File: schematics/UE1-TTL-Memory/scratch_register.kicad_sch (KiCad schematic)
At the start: 9 parts, among them U1 74LS139, U2 74LS259, U3 74LS151, U4 74LS125

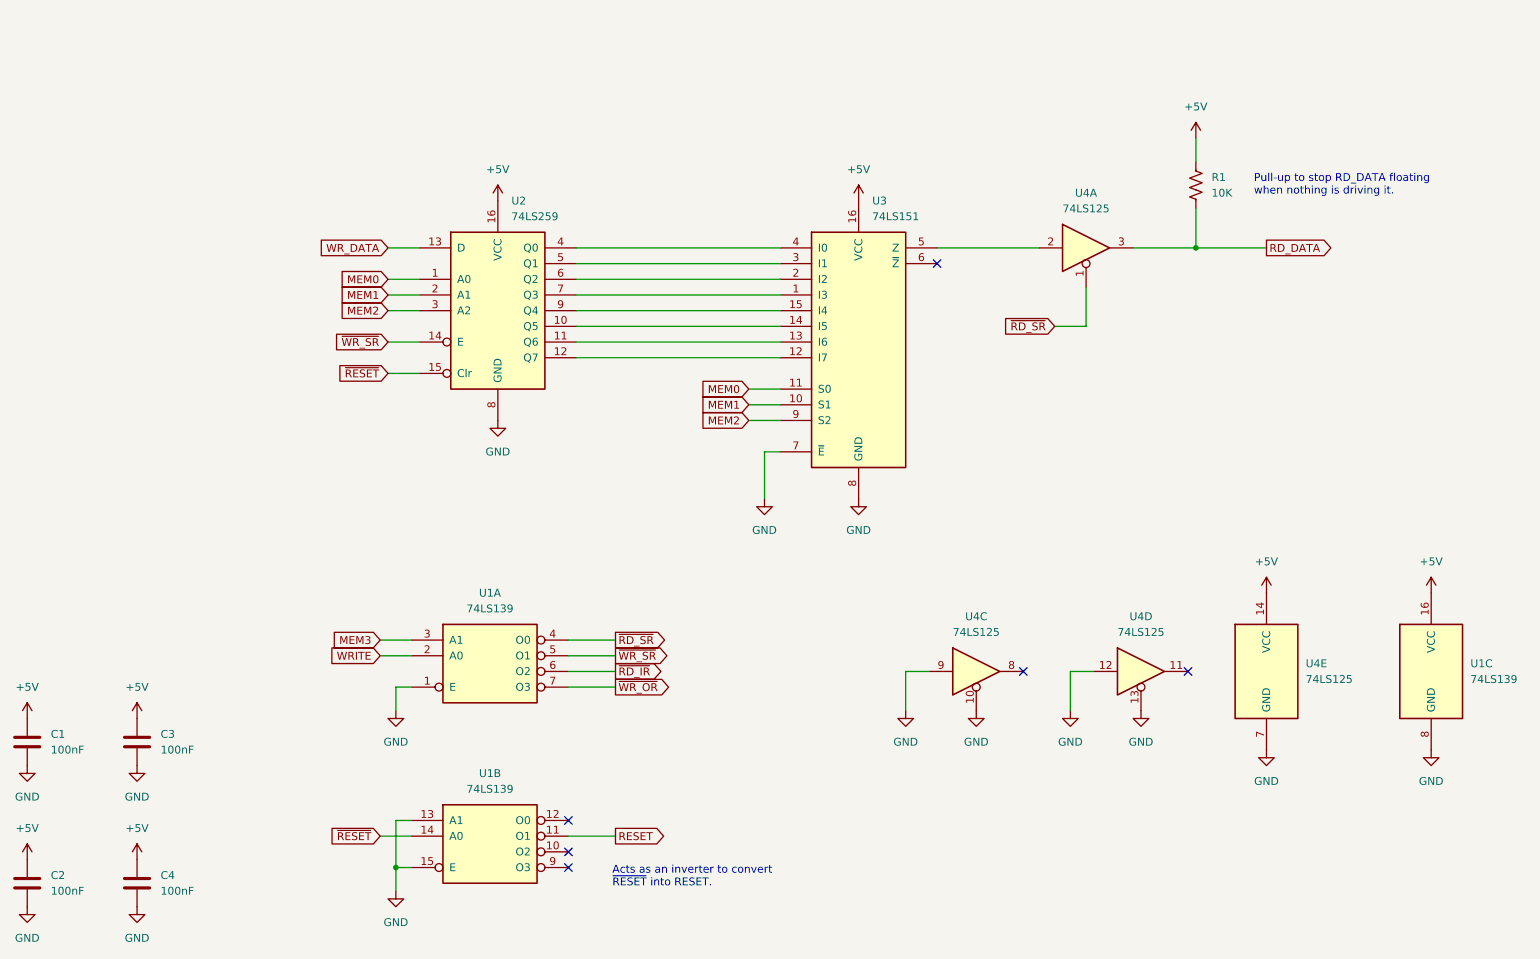
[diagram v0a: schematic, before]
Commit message: Lay out memory board
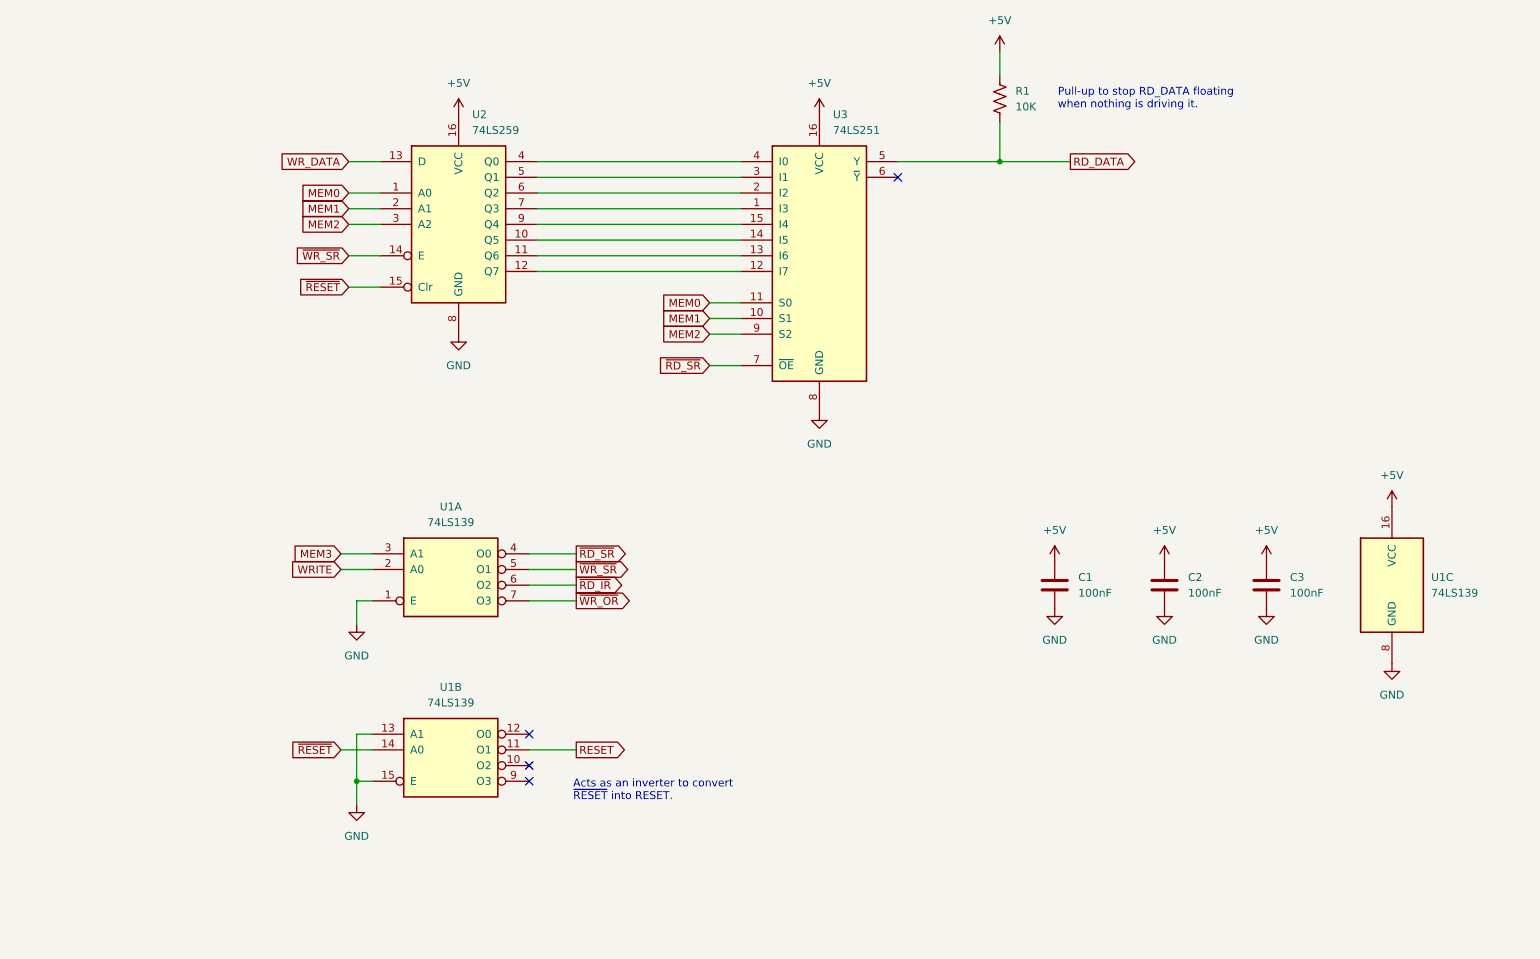
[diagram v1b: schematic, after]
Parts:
- removed C2: 100nF, Capacitor_THT:C_Disc_D5.0mm_W2.5mm_P5.00mm, symbol Device:C
- removed U3: 74LS151, Package_DIP:DIP-16_W7.62mm, symbol 74xx:74LS151
- removed U4: 74LS125, Package_DIP:DIP-14_W7.62mm, symbol 74xx:74LS125
- added U3: 74LS251, Package_DIP:DIP-16_W7.62mm, symbol 74xx:74LS251
- renumbered C4 to C2
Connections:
- net +5V: now also U3.16 (VCC)
- net GND: now also U3.8 (GND)
- net MEM0: now also U3.11 (S0)
- net MEM1: now also U3.10 (S1)
- net MEM2: now also U3.9 (S2)
- net RD_DATA: now also U3.5 (Y)
- net ~{RD_SR}: now also U3.7 (~{OE})
- net at U2.10 (Q5): now also U3.14 (I5)
- net at U2.11 (Q6): now also U3.13 (I6)
- net at U2.12 (Q7): now also U3.12 (I7)
- net at U2.4 (Q0): now also U3.4 (I0)
- net at U2.5 (Q1): now also U3.3 (I1)
- net at U2.6 (Q2): now also U3.2 (I2)
- net at U2.7 (Q3): now also U3.1 (I3)
- net at U2.9 (Q4): now also U3.15 (I4)
- no-connect marks 6 -> 4
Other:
- moved on the sheet: C1, C2, C3, R1, U1A, U1B, U1C, U2
